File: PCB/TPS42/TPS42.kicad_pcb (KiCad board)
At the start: 2 copper layers, 138.1 x 89.7 mm, 77 parts, among them J1 PJ-320A, J11 Conn_01x06, J14 FH12-10S-0.5SH, J3 TP Sensor Module, J4 TP Module, J6 OLED, J7 TrackPoint, J8 Battery, J9 TP Sensor Module, SW1 SW_DPST_x2, SW2 Reset, SW3 Reset, U1 ProMicro, U11 Hole, U12 Hole, U14 ProMicro, U2 Hole, U3 Hole, U4 Hole, U5 Hole, U7 Hole, U8 Hole, U9 Hole

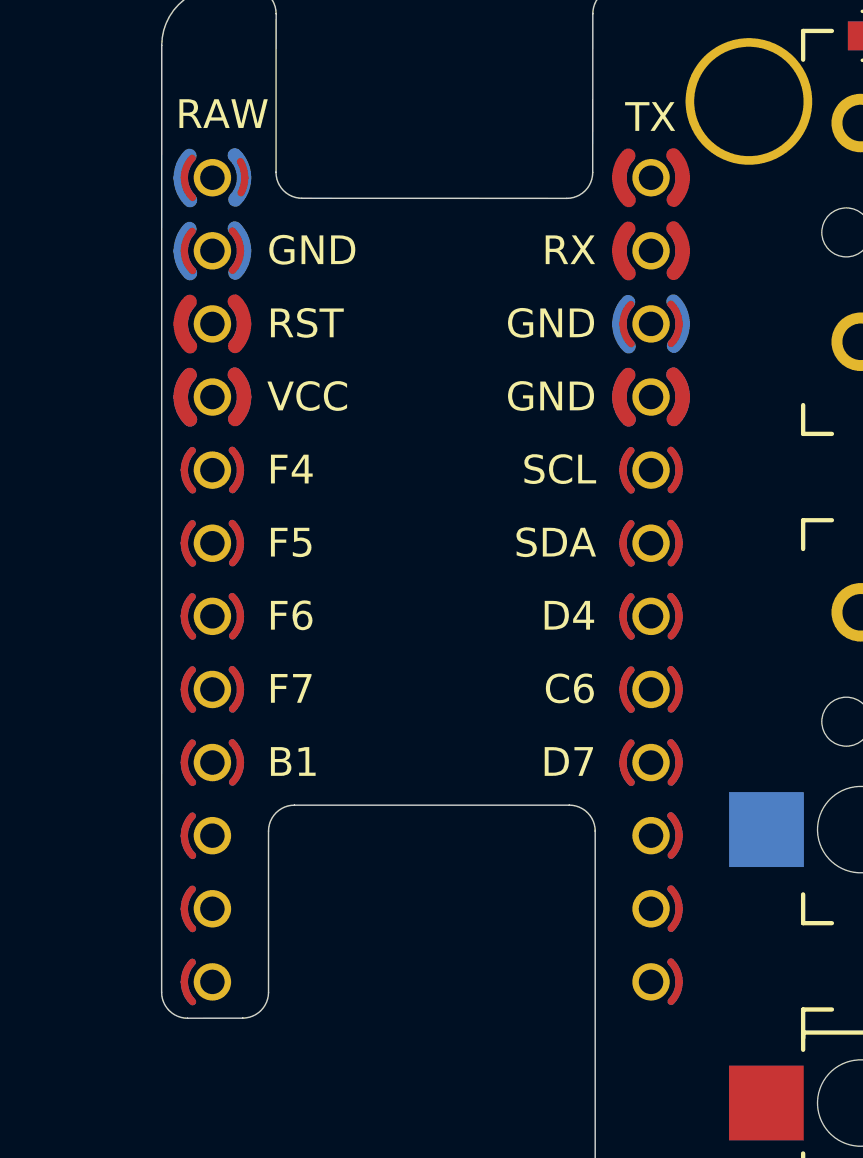
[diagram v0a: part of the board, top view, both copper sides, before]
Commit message: mcu bridges
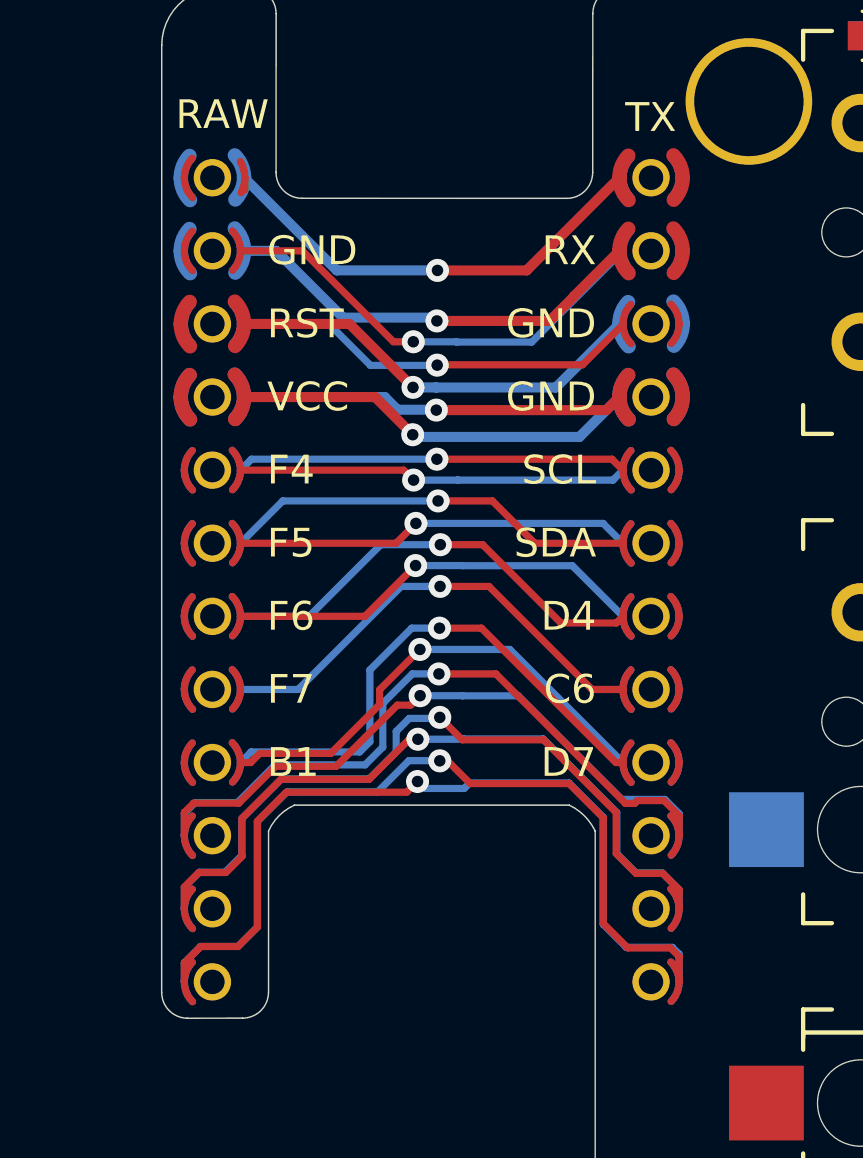
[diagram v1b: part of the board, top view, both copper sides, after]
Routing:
- net GND: track 0.00 -> 44.1 mm, vias 0 -> 3
- net COL3: track 0.00 -> 28.8 mm, vias 0 -> 1
- net COL4: track 0.00 -> 28.4 mm, vias 0 -> 1
- net COL2: track 0.00 -> 25.5 mm, vias 0 -> 1
- net COL5: track 0.00 -> 24.5 mm, vias 0 -> 1
- net COL1: track 0.00 -> 23.7 mm, vias 0 -> 1
- net TP_CLK: track 0.00 -> 22.1 mm, vias 0 -> 1
- net COL0: track 0.00 -> 18.6 mm, vias 0 -> 1
- net TP_DATA: track 0.00 -> 16.8 mm, vias 0 -> 1
- net ROW3: track 0.00 -> 16.3 mm, vias 0 -> 1
- net SERIAL: track 0.00 -> 16.0 mm, vias 0 -> 1
- net BAT+: track 0.00 -> 15.7 mm, vias 0 -> 1
- net ROW2: track 0.00 -> 15.5 mm, vias 0 -> 1
- net CS: track 0.00 -> 14.8 mm, vias 0 -> 1
- net ROW1: track 0.00 -> 14.5 mm, vias 0 -> 1
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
